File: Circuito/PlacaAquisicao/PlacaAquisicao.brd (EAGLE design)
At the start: 149.8 x 88.6 mm, 98 parts, among them IC2 LM7805, IC3 MEGA8-AI, IC4 ACS712-LC, IC5 MEGA8-AI, IC6 ACS712-LC, IC7 MCP602P, IC8 MCP602P, P1 SPI, P2 SPI, Q1 16MHz, X1 MC4-G, X2 MC4-G, X3 MSTBA2, X4 MSTBA2, X6 MC4-G, X7 MC4-G

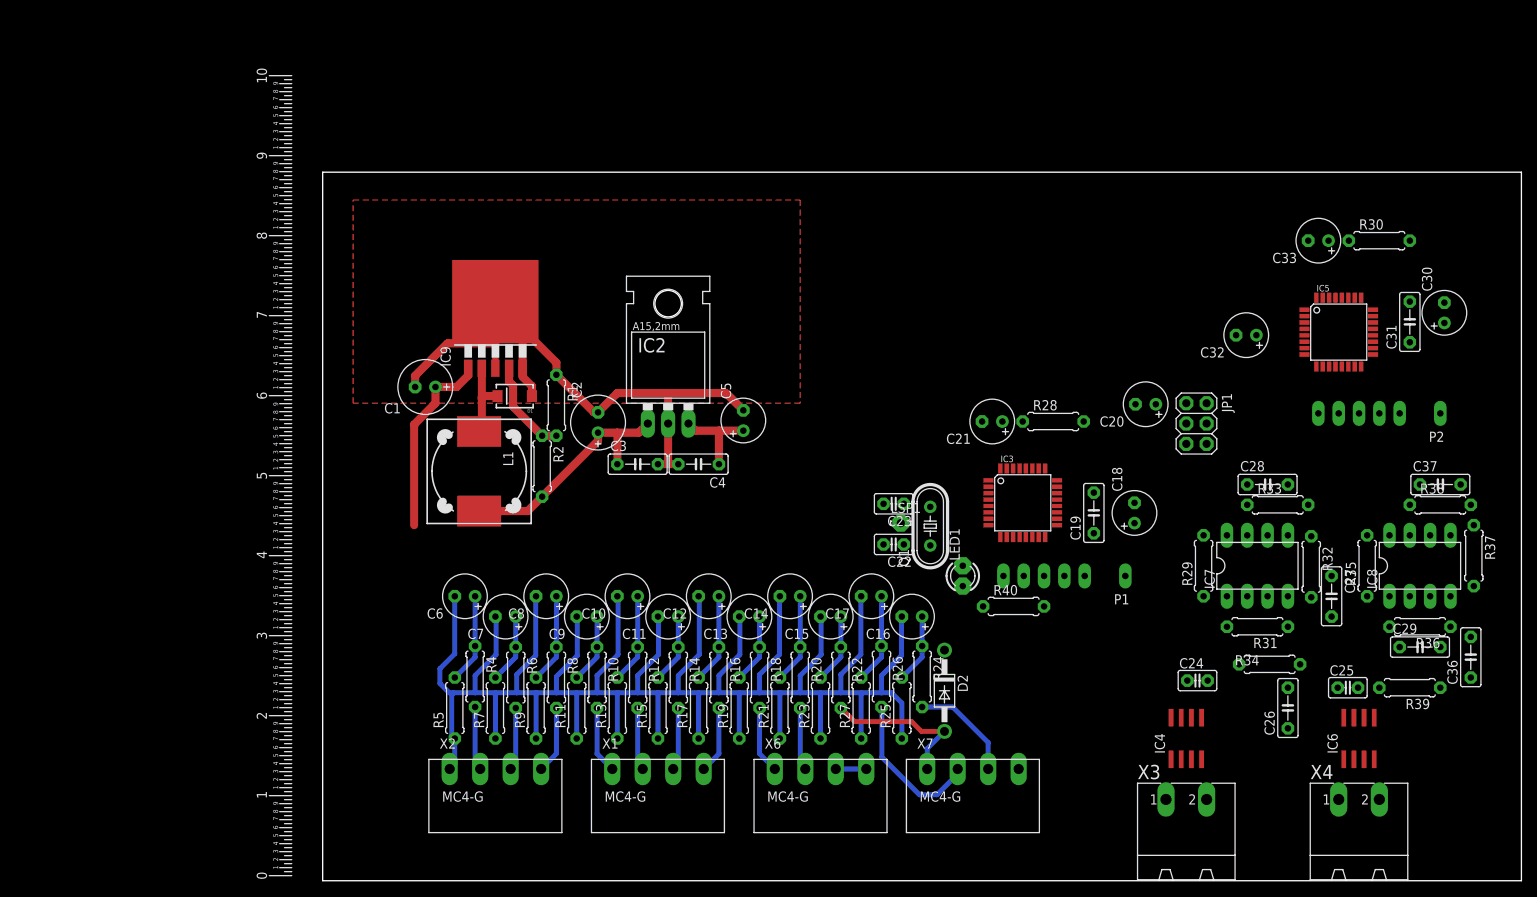
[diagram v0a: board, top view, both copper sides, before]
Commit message: Atualizando...
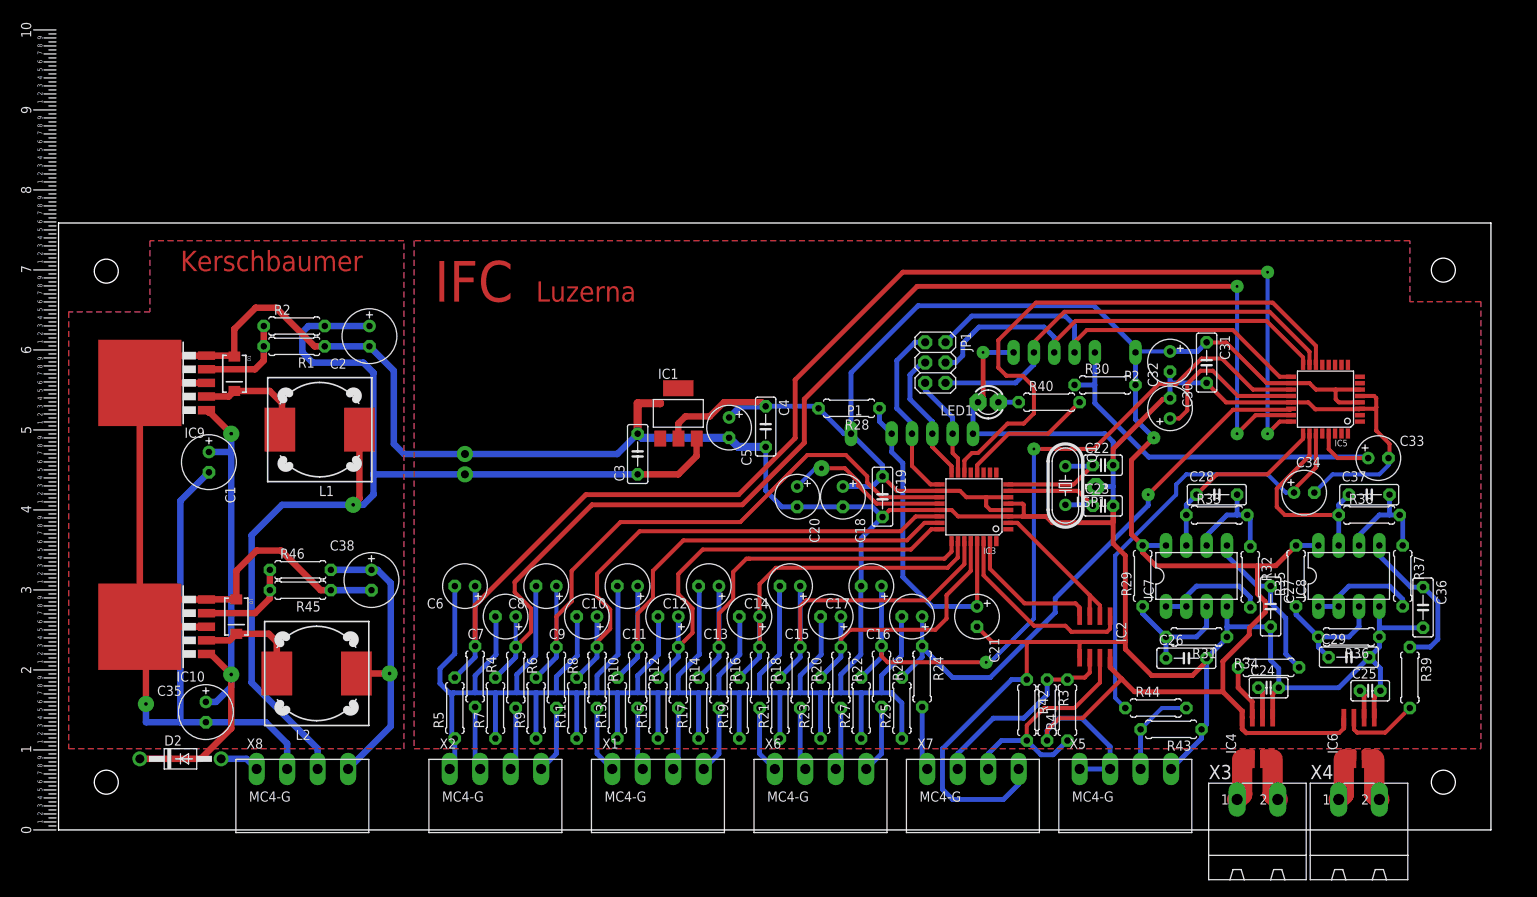
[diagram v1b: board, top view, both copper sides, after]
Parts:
- added C34: 4,7uF, rcl:E2,5-6
- added C35: 100uF 50V, rcl:E2,5-7
- added C38: 470uF 16V, rcl:E2,5-7
- added D3: SS56, ,RK_SteveMarple:SMA-DIODE
- added IC1: REG1117, burr-brown:SOT223
- added IC10: (no value), linear:TO263-5
- added L2: 100uH, inductors:DR125
- added R3, R42: 560, rcl:0207/7
- added R41: 120, rcl:0207/7
- added R43, R45: 1K, rcl:0207/7
- added R44: 10K, rcl:0207/7
- added R46: 11.3K, rcl:0207/7
- added X5, X8: MC4-G, con-phoenix-381_l:MC4-G
- IC2: value LM7805 -> LTC485S; device v-reg:78XXL -> linear-technology:SOIC8
- R10, R12, R14, R16, R18, R20, R22, R24, R26, R4, R6, R8: value 8,3K -> 9,1K
- moved D2 95.9 mm to (-17.8, 15.2), turned to 0 degrees
- moved IC2 61.4 mm to (96.5, 30.5), turned to 180 degrees
- moved C20 45.1 mm to (59.3, 48.0), turned to 270 degrees
- moved IC9 42.6 mm to (-20.3, 62.2), turned to 90 degrees
- moved P2 38.9 mm to (94.0, 66.0)
- moved R30 38.7 mm to (97.8, 62.0)
- moved C18 36.5 mm to (65.0, 48.0), turned to 270 degrees
- moved R2 35.6 mm to (-3.56, 69.3), turned to 0 degrees
- moved D1 35.2 mm to (-11.0, 63.4), turned to 270 degrees
- moved C30 34.8 mm to (105.9, 64.9), turned to 270 degrees
- moved R1 33.6 mm to (-3.56, 66.8), turned to 180 degrees
- moved JP1 33.5 mm to (76.6, 64.8)
- moved C2 30.5 mm to (5.84, 68.1), turned to 270 degrees
- moved U$1 30.0 mm to (-34.0, 6.35)
- moved C1 28.6 mm to (-14.2, 52.3), turned to 270 degrees
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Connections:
- removed net N$20: R26.2, X7.2
- new net +15V: C38.+, L2.2, R46.2, X8.4
- new net N$35: R43.2, R44.2, X5.3
- new net N$36: IC10.4, R45.2, R46.1
- new net N$37: D3.C, IC10.2, L2.1
- new net N$5: IC3.14, IC5.14
- new net RS485A: IC2.6, R3.1, R41.2, X7.2
- new net RS485B: IC2.7, R41.1, R42.2, X7.3
- new net RXD: IC2.1, IC3.30
- new net TEMP_IN: C34.+, IC5.27, R44.1
- new net TXD: IC2.4, IC3.31
- new net TXE: IC2.2, IC2.3, IC3.2
- new net VC10: R22.2, X6.3
- net +5V: now also IC1.2, IC2.8, R3.2, X5.1, X5.2; no longer IC2.OUT
- net +8V: now also IC1.3, X8.3; no longer IC2.IN
- net ADC0A: now also C10.+, R12.1, R13.2; no longer C13.+, R18.1, R19.2
- net ADC1A: now also C11.+, R14.1, R15.2; no longer C12.+, R16.1, R17.2
- net ADC2A: now also C12.+, R16.1, R17.2; no longer C11.+, R14.1, R15.2
- net ADC3A: now also C13.+, R18.1, R19.2; no longer C10.+, R12.1, R13.2
- net ADC4A: now also C14.+, R20.1, R21.2; no longer C9.+, R10.1, R11.2
- net ADC5A: now also C15.+, R22.1, R23.2; no longer C8.+, R8.1, R9.2
- net ADC6A: now also C8.+, R8.1, R9.2; no longer C15.+, R22.1, R23.2
- net ADC7A: now also C9.+, R10.1, R11.2; no longer C14.+, R20.1, R21.2
- net GND: now also C34.-, C35.-, C38.-, D3.A, IC1.1, IC10.3, IC10.5, IC10.6, IC2.5, R42.1, R43.1, R45.1, X5.4, X7.4, X8.2; no longer IC2.GND
- net N$1: now also C35.+, IC10.1
- net N$10: now also R26.2; no longer X6.3
- net N$11: now also X4.2; no longer X4.1
- net N$12: now also X4.1; no longer X4.2
- net N$18: now also X3.1; no longer X3.2
- net N$21: now also X7.1; no longer X7.3
- net N$33: now also JP1.4; no longer JP1.6
- net N$34: now also JP1.6; no longer JP1.4
- net N$9: now also X3.2; no longer X3.1
- net VIN: now also X8.1; no longer R22.2, X7.1
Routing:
- net GND: track 355.7 -> 878.1 mm, vias 0 -> 3
- net +5V: track 11.4 -> 290.0 mm, vias 0 -> 1
- net ADC1B: track 11.2 -> 161.9 mm, vias 0 -> 2
- net ADC0B: track 8.67 -> 153.4 mm, vias 0 -> 2
- net +8V: track 30.1 -> 139.6 mm, vias 0 -> 2
- net ADC6B: track 11.2 -> 95.0 mm, vias 0 -> 2
- net N$5: track 0.00 -> 71.1 mm
- net ADC6A: track 8.67 -> 77.4 mm
- net ADC7B: track 8.67 -> 72.1 mm, vias 0 -> 1
- net TEMP_IN: track 0.00 -> 56.4 mm
- net N$33: track 0.00 -> 55.0 mm
- net N$34: track 0.00 -> 54.5 mm
- net ADC7A: track 11.2 -> 65.0 mm
- net N$17: track 0.00 -> 53.2 mm
- net N$32: track 0.00 -> 52.7 mm
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- added copper zone on layer 16, net GND
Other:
- board size 149.8 x 88.6 mm -> 179.1 x 75.9 mm
- board text added: "IFC"
- board text added: "Kerschbaumer"
- board text added: "Luzerna"
